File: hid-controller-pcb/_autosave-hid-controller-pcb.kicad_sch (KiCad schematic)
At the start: 65 parts, among them IC1 RT9080-33GJ5, J1 10118194-0011LF, J2 Jumper, J3 STLink, U1 STM32F103C8Tx, U3 COM-09032, U4 COM-09032, Y1 8MHz, Y2 32.768KHz

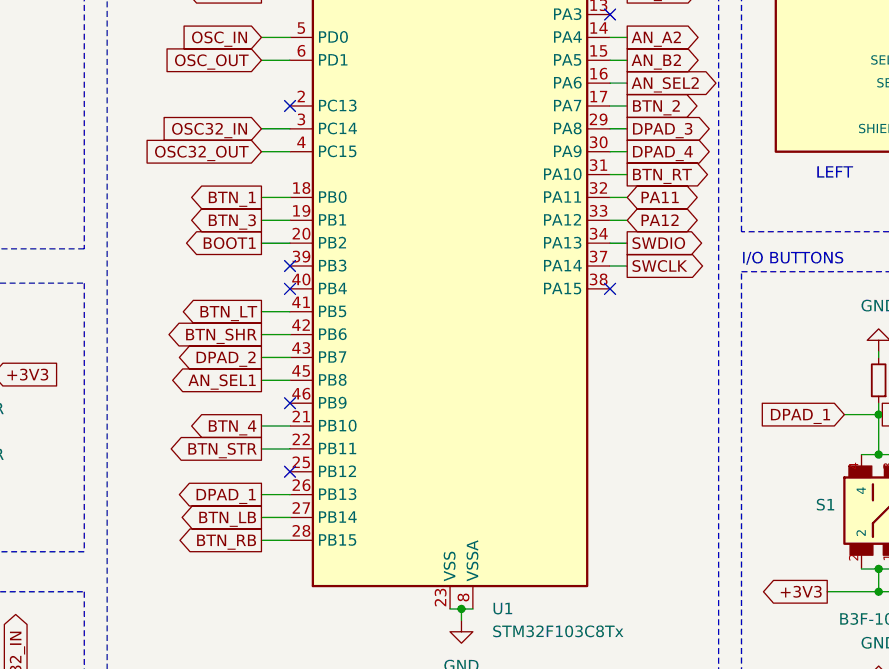
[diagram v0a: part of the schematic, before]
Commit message: further work on controller
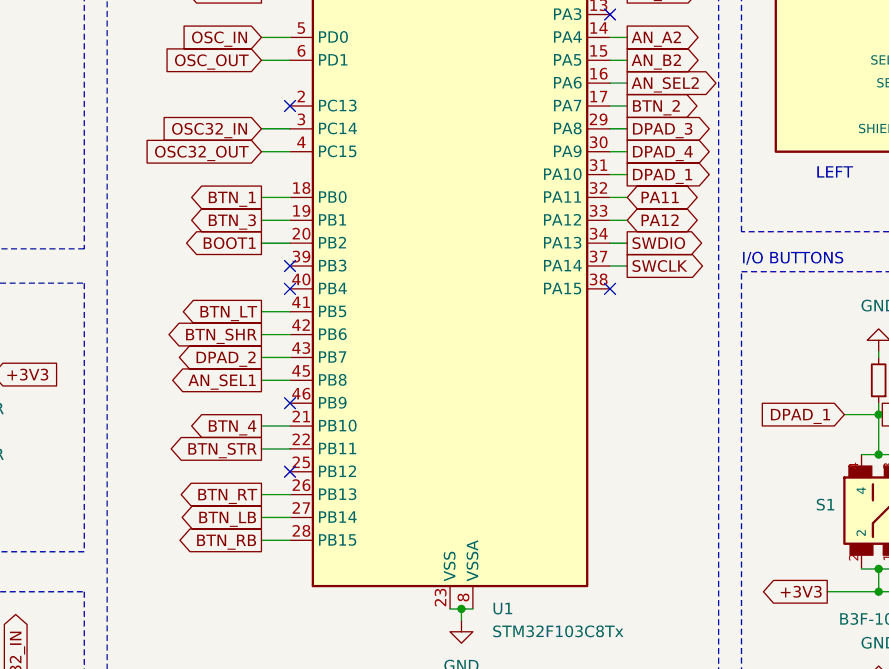
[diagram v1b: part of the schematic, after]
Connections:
- net BTN_RT: now also U1.26 (PB13); no longer U1.31 (PA10)
- net DPAD_1: now also U1.31 (PA10); no longer U1.26 (PB13)
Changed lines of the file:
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@@
 	(global_label "DPAD_1"
 		(shape output)
-		(at 93.98 97.155 180)
-		(fields_autoplaced yes)
-		(effects
-			(font
-				(size 1.27 1.27)
-			)
-			(justify right)
-		)
-		(property "Intersheetrefs" "${INTERSHEET_REFS}"
-			(at 84.8224 97.155 0)
-			(hide yes)
-			(show_name no)
-			(do_not_autoplace no)
-			(effects
-				(font
-					(size 1.27 1.27)
-				)
-				(justify right)
+		(at 134.62 61.595 0)
+		(fields_autoplaced yes)
+		(effects
+			(font
+				(size 1.27 1.27)
+			)
+			(justify left)
+		)
+		(property "Intersheetrefs" "${INTERSHEET_REFS}"
+			(at 143.7776 61.595 0)
+			(hide yes)
+			(show_name no)
+			(do_not_autoplace no)
+			(effects
+				(font
+					(size 1.27 1.27)
+				)
+				(justify left)
 			)
 		)
@@
 	(global_label "BTN_RT"
 		(shape output)
-		(at 134.62 61.595 0)
-		(fields_autoplaced yes)
-		(effects
-			(font
-				(size 1.27 1.27)
-			)
-			(justify left)
-		)
-		(property "Intersheetrefs" "${INTERSHEET_REFS}"
-			(at 143.7776 61.595 0)
-			(hide yes)
-			(show_name no)
-			(do_not_autoplace no)
-			(effects
-				(font
-					(size 1.27 1.27)
-				)
-				(justify left)
-			)
-		)
+		(at 93.98 97.155 180)
+		(fields_autoplaced yes)
+		(effects
+			(font
+				(size 1.27 1.27)
+			)
+			(justify right)
+		)
+		(property "Intersheetrefs" "${INTERSHEET_REFS}"
+			(at 84.8224 97.155 0)
+			(hide yes)
+			(show_name no)
+			(do_not_autoplace no)
+			(effects
+				(font
+					(size 1.27 1.27)
+				)
+				(justify right)
+			)
+		)
